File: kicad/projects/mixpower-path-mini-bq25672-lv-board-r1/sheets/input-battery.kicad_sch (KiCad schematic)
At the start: 13 parts, among them J2 BAT_HEADERS, J3 BATT, Q4 DMN3032LFDBQ, U4 MAX17055ETB

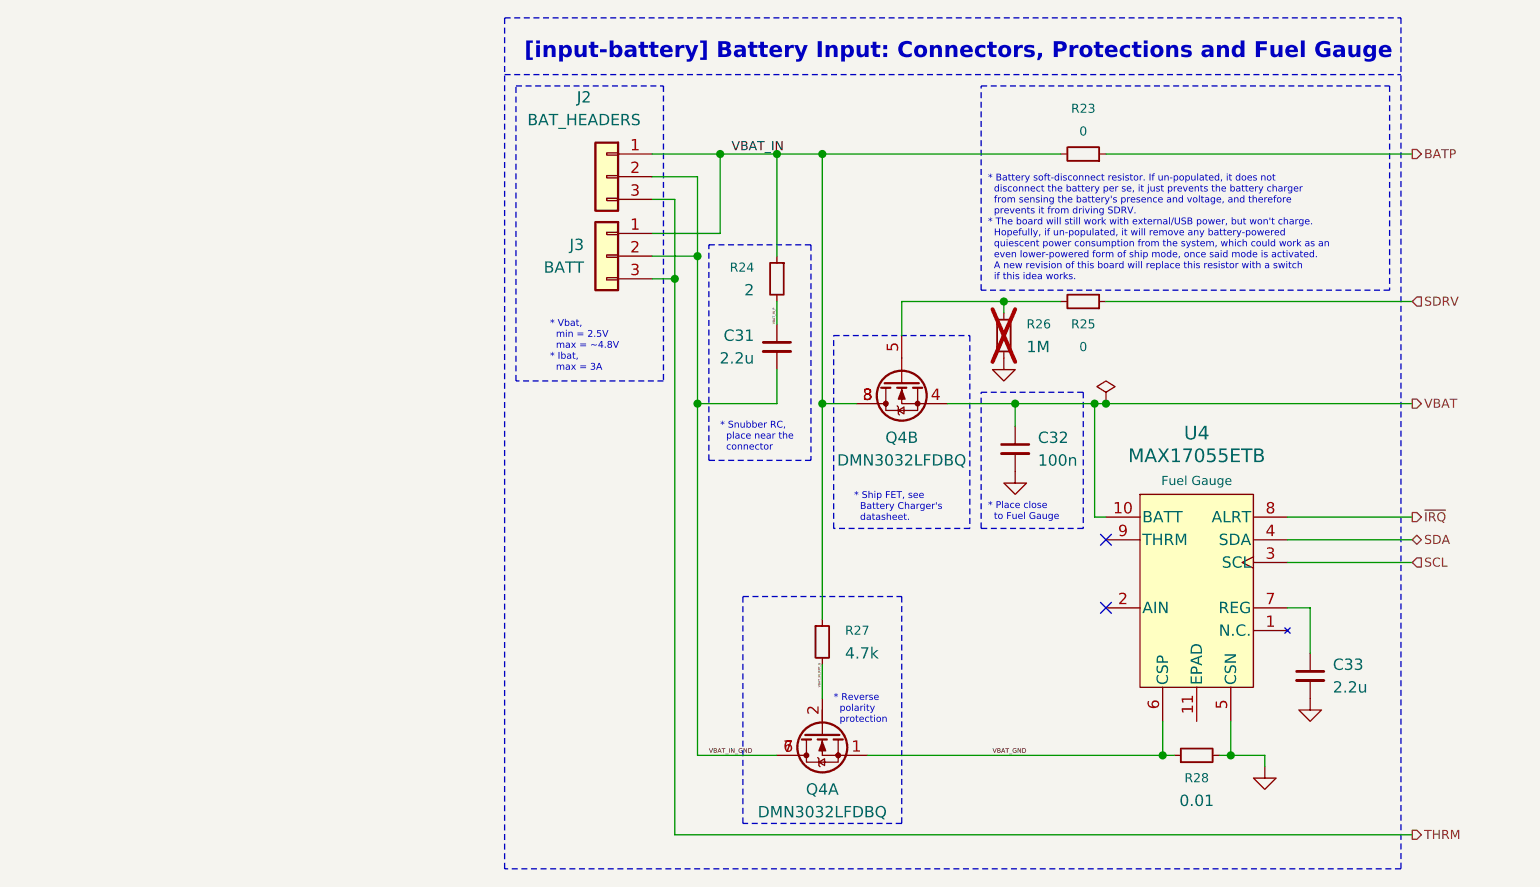
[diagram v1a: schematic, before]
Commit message: feat: failed PCB routing
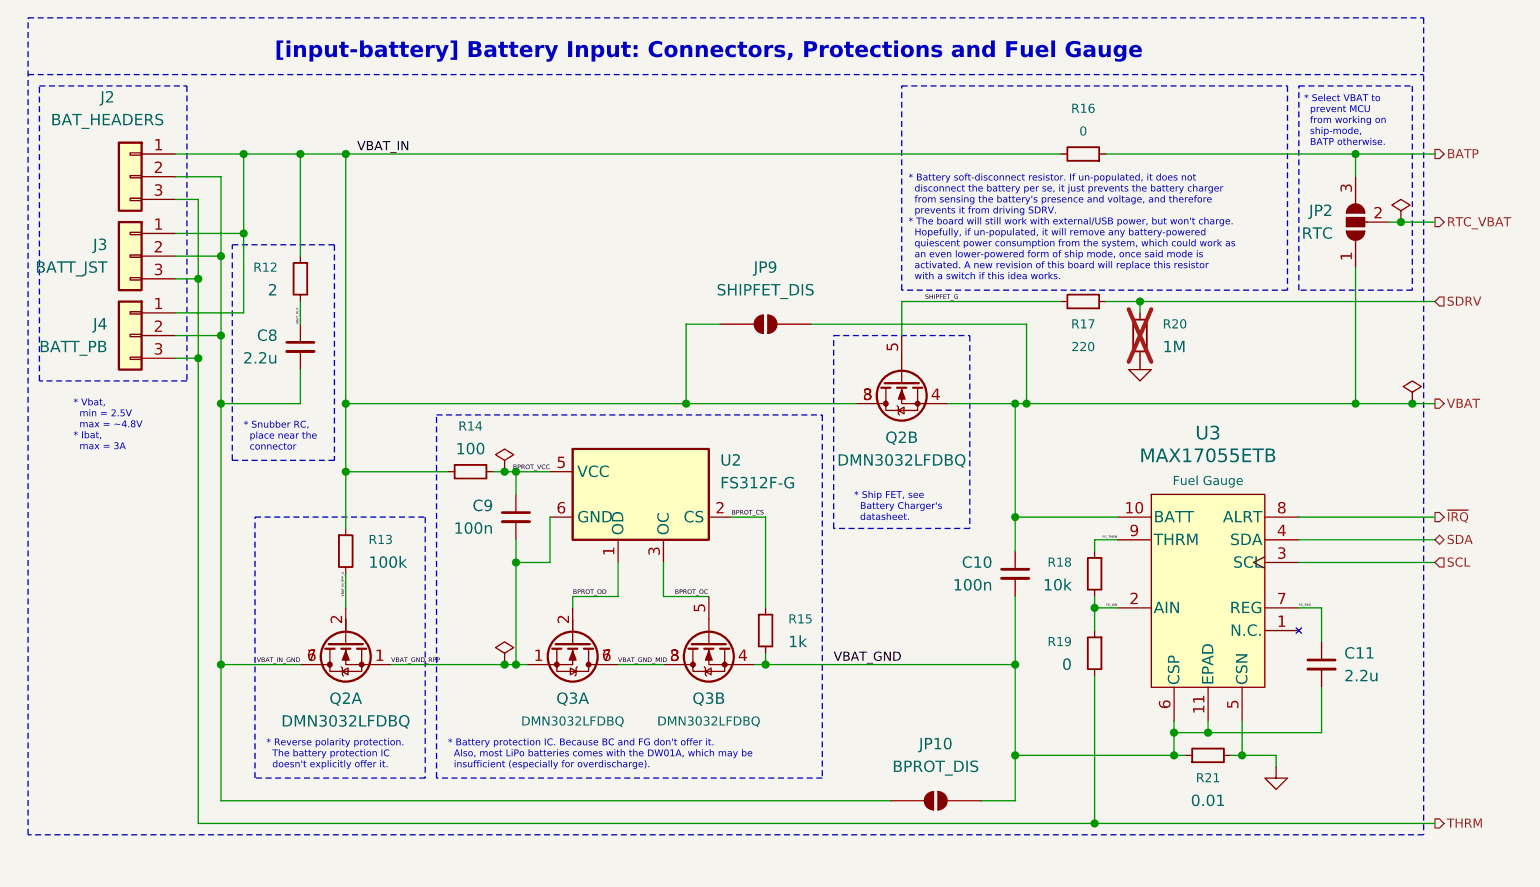
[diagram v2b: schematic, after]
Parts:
- removed C32: 100n, Capacitor_SMD:C_0402_1005Metric, symbol Device:C_Small
- removed R25: 0, Resistor_SMD:R_0402_1005Metric, symbol Device:R_Small
- added C10, C9: 100n, Capacitor_SMD:C_0402_1005Metric, symbol Device:C_Small
- added J4: BATT_PB, Connector_Molex:Molex_PicoBlade_53048-0310_1x03_P1.25mm_Horizontal, symbol Connector_Generic:Conn_01x03
- added JP10: BPROT_DIS, Jumper:SolderJumper-2_P1.3mm_Open_Pad1.0x1.5mm, symbol Jumper:SolderJumper_2_Open
- added JP2: RTC, Jumper:SolderJumper-3_P1.3mm_Open_Pad1.0x1.5mm, symbol Jumper:SolderJumper_3_Open
- added JP9: SHIPFET_DIS, Jumper:SolderJumper-2_P1.3mm_Open_Pad1.0x1.5mm, symbol Jumper:SolderJumper_2_Open
- added Q3: DMN3032LFDBQ, mixlib-generic-dfn:Diodes-Incorporated_U-DFN2020-6_Type-B, symbol mixlib-discrete-mosfet:DMN3032LFDBQ
- added R14: 100, Resistor_SMD:R_0402_1005Metric, symbol Device:R_Small
- added R15: 1k, Resistor_SMD:R_0402_1005Metric, symbol Device:R_Small
- added R17: 220, Resistor_SMD:R_0402_1005Metric, symbol Device:R_Small
- added R18: 10k, Resistor_SMD:R_0402_1005Metric, symbol Device:R_Small
- added R19: 0, Resistor_SMD:R_0402_1005Metric, symbol Device:R_Small
- added U2: FS312F-G, Package_TO_SOT_SMD:SOT-23-6, symbol Battery_Management:DW01A
- C8: renamed from C31; footprint Capacitor_SMD:C_0603_1608Metric -> Capacitor_SMD:C_0402_1005Metric
- J3: value BATT -> BATT_JST
- R13: renamed from R27; value 4.7k -> 100k
- R21: renamed from R28; footprint Resistor_SMD:R_1210_3225Metric -> Resistor_SMD:R_1206_3216Metric
- renumbered C33 to C11, Q4 to Q2, R24 to R12, R23 to R16, R26 to R20, U4 to U3
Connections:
- net BATP: now also JP2.3 (B)
- net GND: no longer C11.2
- net SDRV: now also R20.1, R17.1
- net THRM: now also J4.3 (Pin_3), R19.2
- net VBAT: now also C10.1, JP2.1 (A), JP9.2 (B)
- net VBAT_GND: now also C11.2, U3.11 (EPAD), C10.2, JP10.2 (B), Q3.4 (S2), R15.2; no longer Q2.1 (S1)
- net VBAT_IN: now also J4.1 (Pin_1), JP9.1 (A), R14.1
- net VBAT_IN_GND: now also J4.2 (Pin_2), JP10.1 (A)
- net FG_REG: now reaches C11.1, U3.7 (REG)
- net SHIPFET_G: now reaches Q2.5 (G2)
- net SHIPFET_G: now also R17.2; no longer R20.1
- net FG_AIN: now reaches U3.2 (AIN)
- net FG_AIN: now also R18.2, R19.1
- net FG_THRM: now reaches U3.9 (THRM)
- net FG_THRM: now also R18.1
- new net BPROT_CS: R15.1, U2.2 (CS)
- new net BPROT_OC: Q3.5 (G2), U2.3 (OC)
- new net BPROT_OD: Q3.2 (G1), U2.1 (OD)
- new net BPROT_VCC: C9.1, R14.2, U2.5 (VCC)
- new net RTC_VBAT: JP2.2 (C)
- new net VBAT_GND_MID: Q3.3 (D2), Q3.6 (D1), Q3.7 (D1), Q3.8 (D2)
- new net VBAT_GND_RPP: C9.2, Q2.1 (S1), Q3.1 (S1), U2.6 (GND)
- no-connect marks 2 -> 0
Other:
- note added: "* Battery protection IC. Because BC and FG don't offer it. Also, most LiPo batteries comes with the DW01A, which may be insufficient (especially for overdischarge)."
- note added: "* Reverse polarity protection. The battery protection IC doesn't explicitly offer it."
- note added: "* Select VBAT to prevent MCU from working on ship-mode, BATP otherwise."
- note removed: "* Place close to Fuel Gauge"
- note removed: "* Reverse polarity protection"
- moved on the sheet: C11, C8, J2, J3, Q2A, R12, R13, R20, R21, U3
